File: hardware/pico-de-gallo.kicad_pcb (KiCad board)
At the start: 4 copper layers, 50 x 69.5 mm, 14 parts, among them J1 Conn_02x08_Odd_Even, J2 Conn_01x02, J3 Conn_01x04, J4 Conn_01x05, J5 Conn_01x02, J6 Conn_01x03, J7 Conn_02x05_Odd_Even

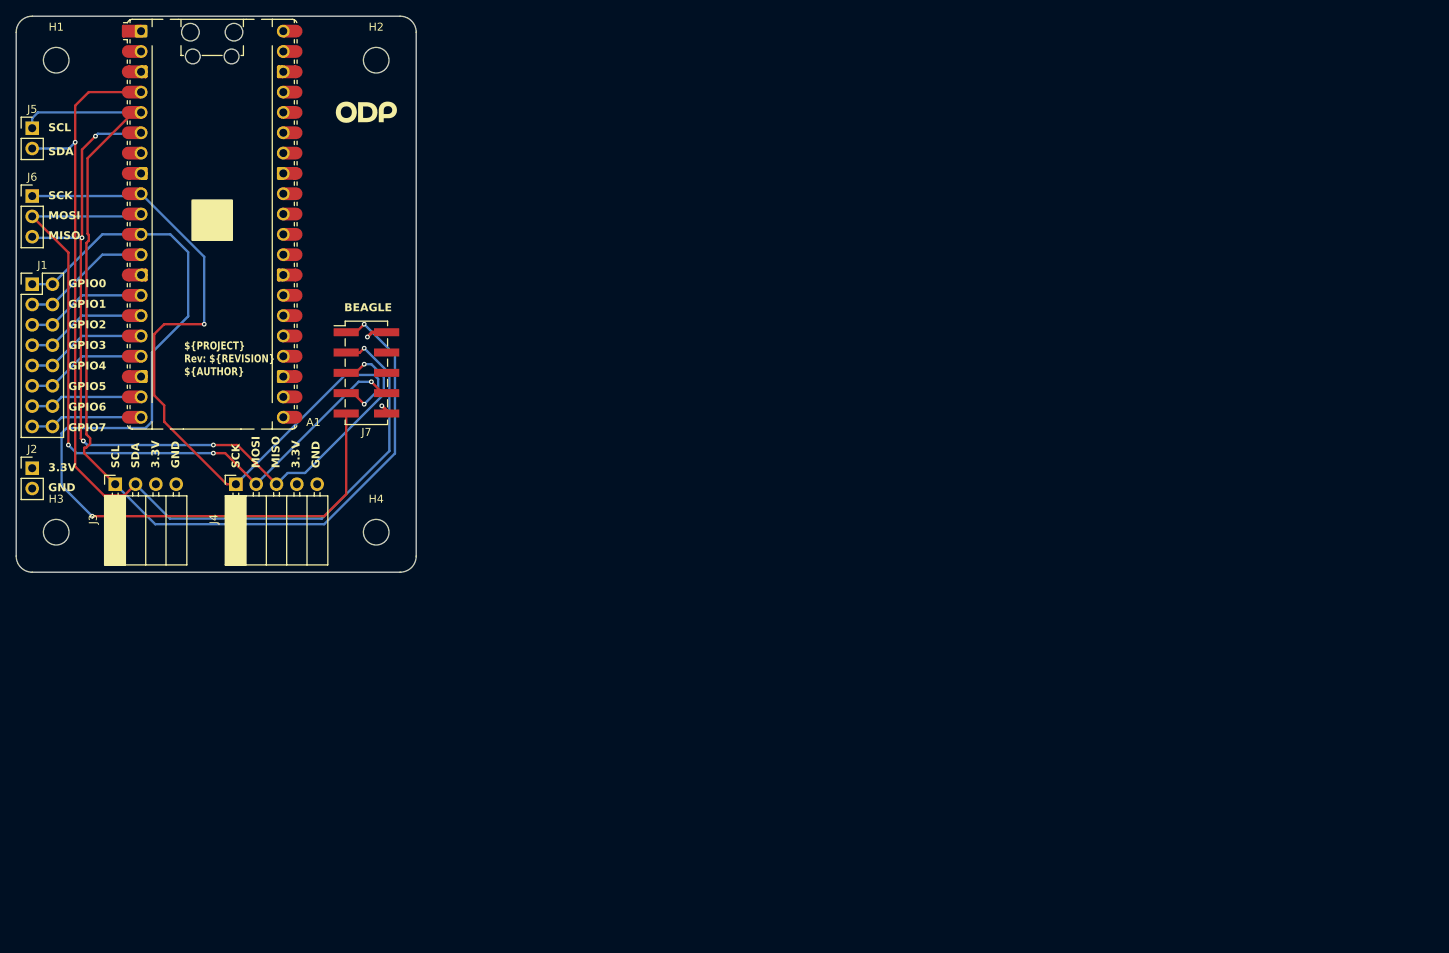
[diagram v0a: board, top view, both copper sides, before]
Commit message: Minor updates
Signed-off-by: Felipe Balbi <febalbi@microsoft.com>
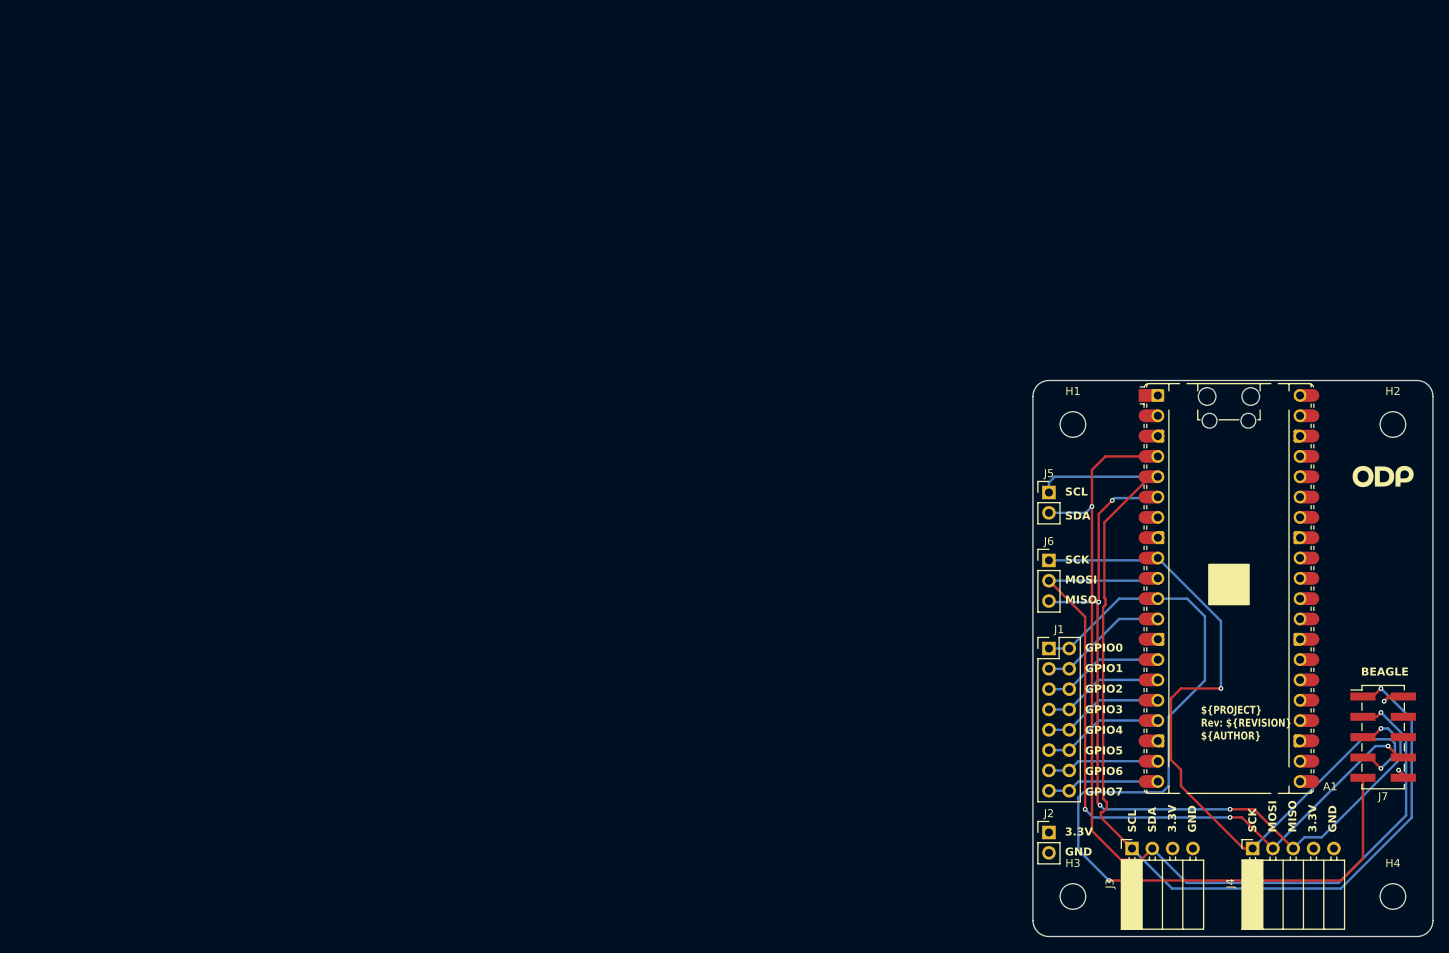
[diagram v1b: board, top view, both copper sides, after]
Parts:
- moved A1 135.0 mm to (152.1, 72.0)
- moved H1 135.0 mm to (132.6, 51.5)
- moved H2 135.0 mm to (172.6, 51.5)
- moved H3 135.0 mm to (132.6, 110.5)
- moved H4 135.0 mm to (172.6, 110.5)
- moved J1 135.0 mm to (129.6, 79.5)
- moved J2 135.0 mm to (129.6, 102.5)
- moved J3 135.0 mm to (140.0, 104.5)
- moved J4 135.0 mm to (155.1, 104.5)
- moved J5 135.0 mm to (129.6, 60.0)
- moved J6 135.0 mm to (129.6, 68.5)
- moved J7 135.0 mm to (171.4, 90.6)
- moved REF** 135.0 mm to (172.9, 81.8)
- moved REF** 135.0 mm to (170.1, 96.5)
